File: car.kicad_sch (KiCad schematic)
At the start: 3 parts, among them SW1 Push_Button

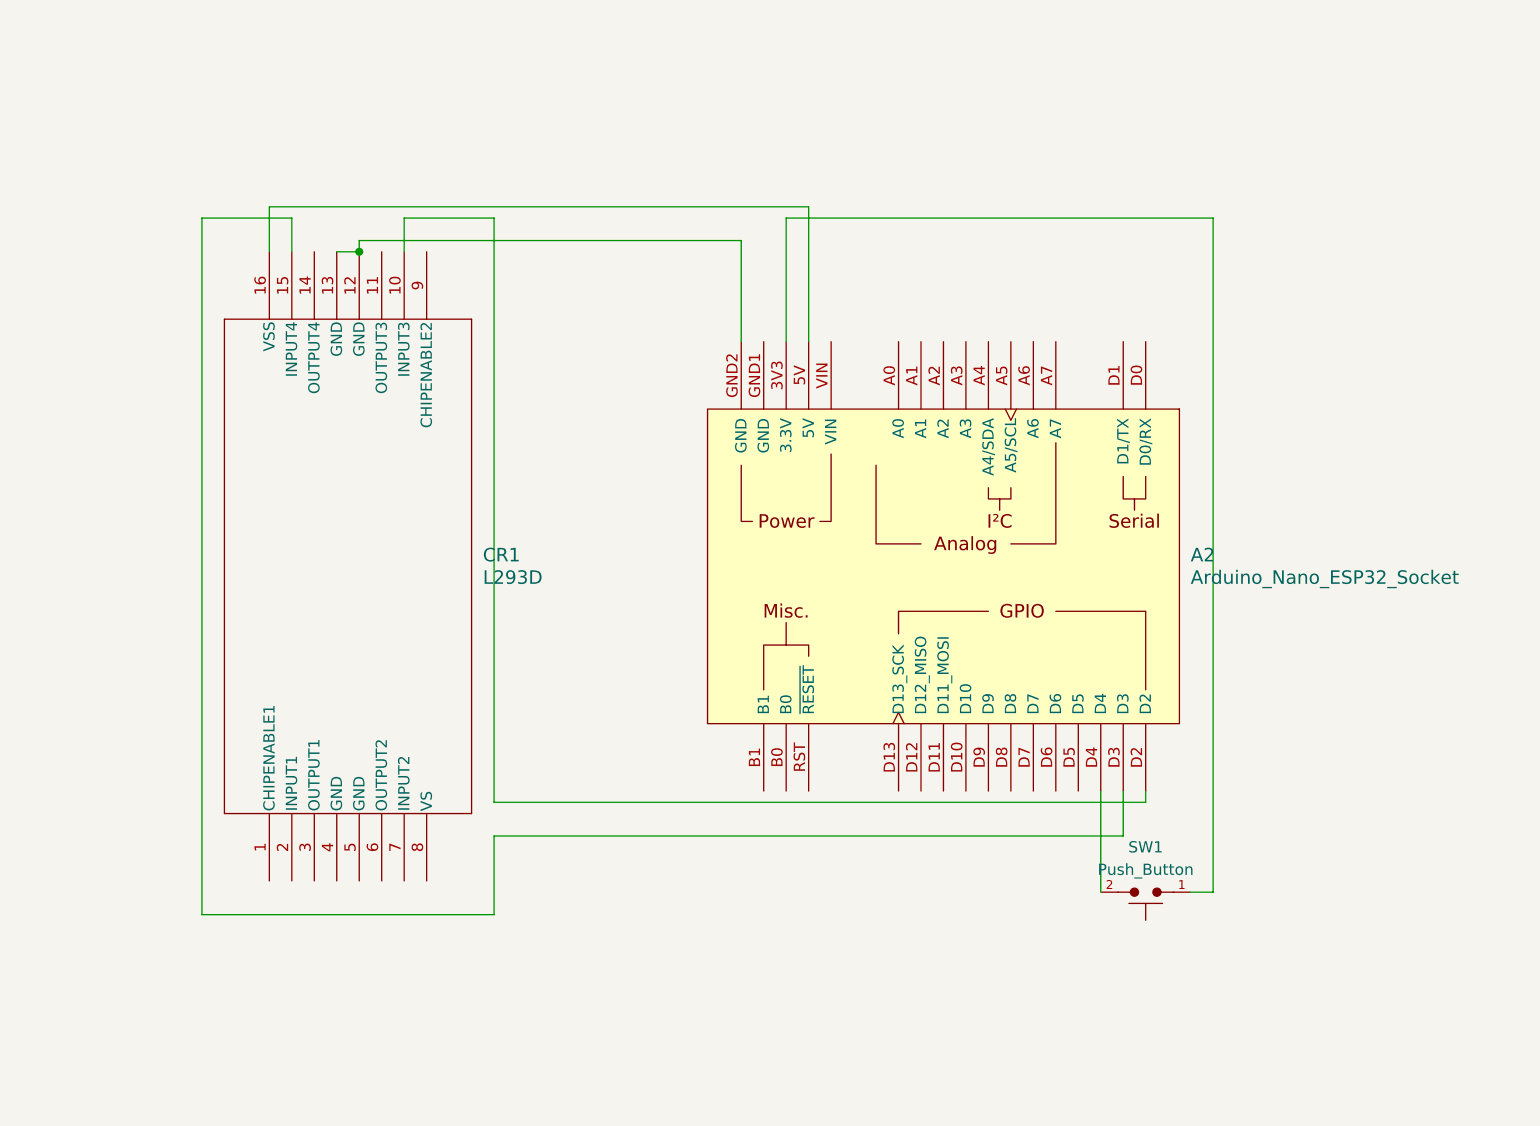
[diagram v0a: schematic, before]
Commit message: add car
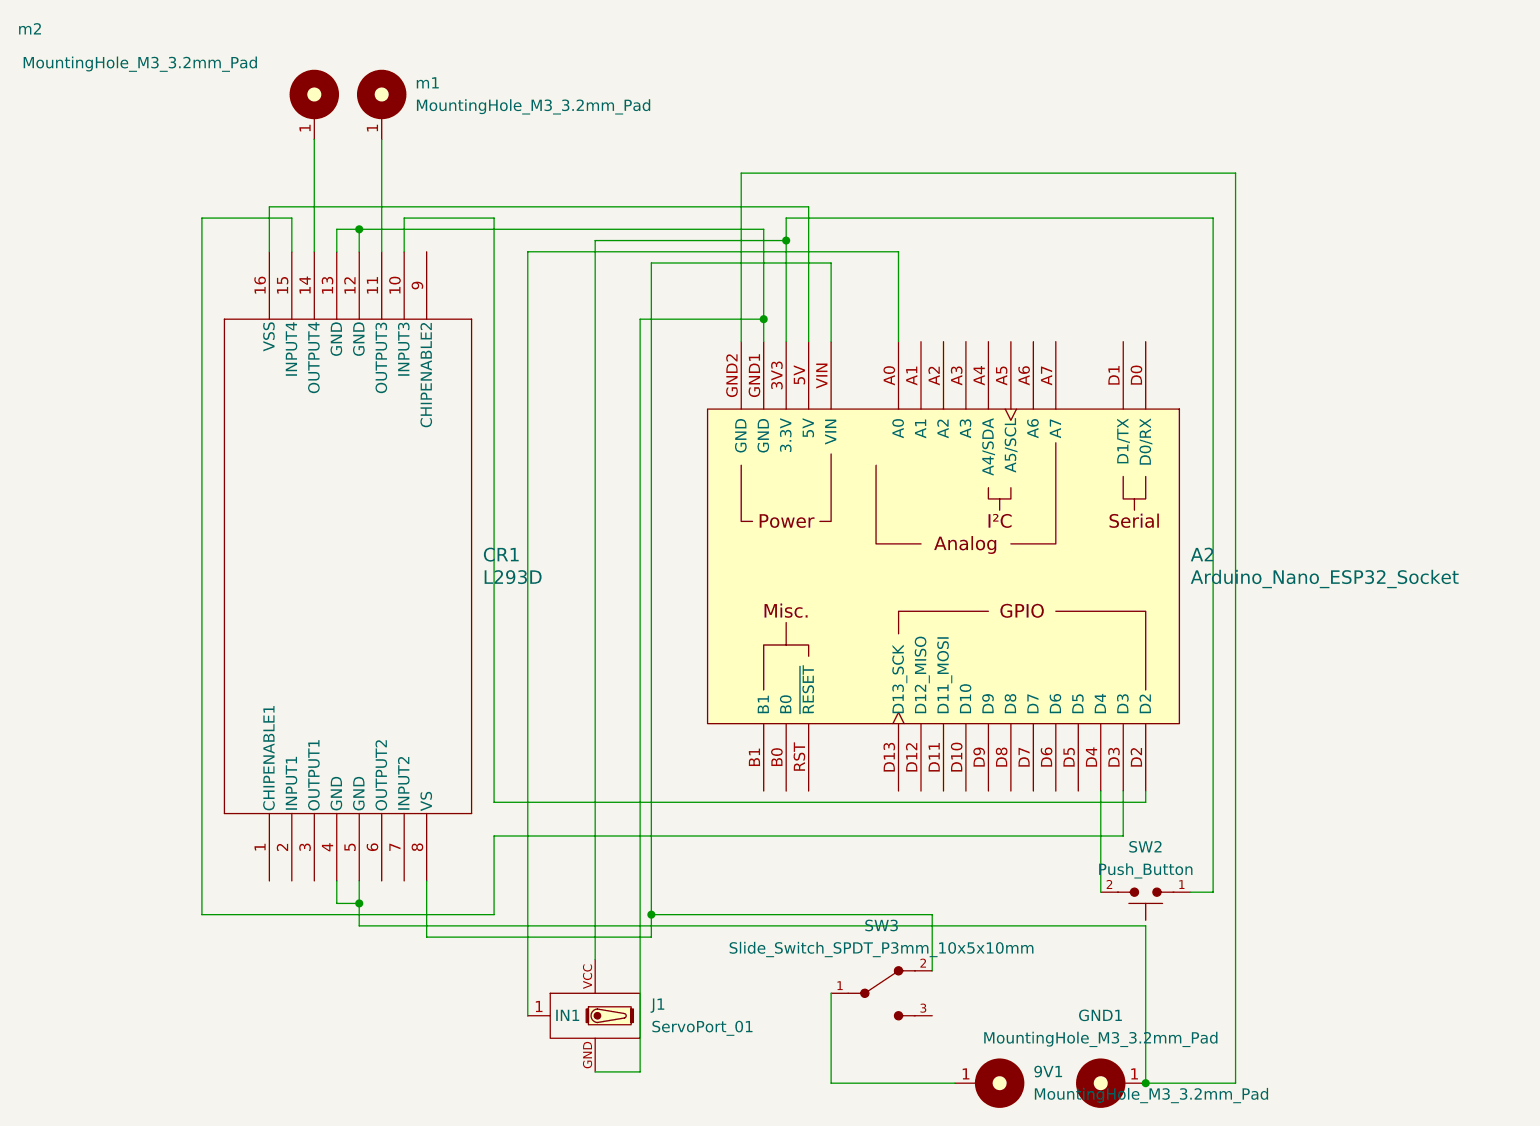
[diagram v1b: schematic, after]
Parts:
- removed SW1: Push_Button, PCM_4ms_Switch:Button_PB20B, symbol PCM_SL_Devices:Push_Button
- added 9V1, GND1, m1, m2: MountingHole_M3_3.2mm_Pad, PCM_SL_Mechanical:MountingHole_3.2mm_Pad, symbol PCM_SL_Mechanical:MountingHole_M3_3.2mm_Pad
- added J1: ServoPort_01, PCM_SL_Connectors:ServoPort_01_Vertical, symbol PCM_SL_Connectors:ServoPort_01
- added SW2: Push_Button, Button_Switch_THT:SW_PUSH_6mm, symbol PCM_SL_Devices:Push_Button
- added SW3: Slide_Switch_SPDT_P3mm_10x5x10mm, PCM_SL_Devices:Slide_Switch_SPDT_P3mm_10x5x10mm, symbol PCM_SL_Devices:Slide_Switch_SPDT_P3mm_10x5x10mm
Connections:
- net at A2.3V3 (3.3V): now also J1.VCC, SW2.1
- net at A2.D4: now also SW2.2
- net at A2.A0: now also J1.1 (IN1)
- net at A2.GND1 (GND): now also CR1.12 (GND), CR1.13 (GND), J1.GND
- net at A2.VIN: now also CR1.8 (VS), SW3.2
- net at CR1.11 (OUTPUT3): now also m1.1
- net at CR1.14 (OUTPUT4): now also m2.1
- net at CR1.4 (GND): now also A2.GND2 (GND), CR1.5 (GND), GND1.1
- new net: 9V1.1, SW3.1
